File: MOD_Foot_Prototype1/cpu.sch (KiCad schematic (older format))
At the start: 19 parts, among them CN1 CONN_PANNEL_2X2, CN2 CONN_PANNEL_2X2, P1 HEADER_5X2, P2 HEADER_5X2, U1 LPC111X_LQFP48, X1 10MHz

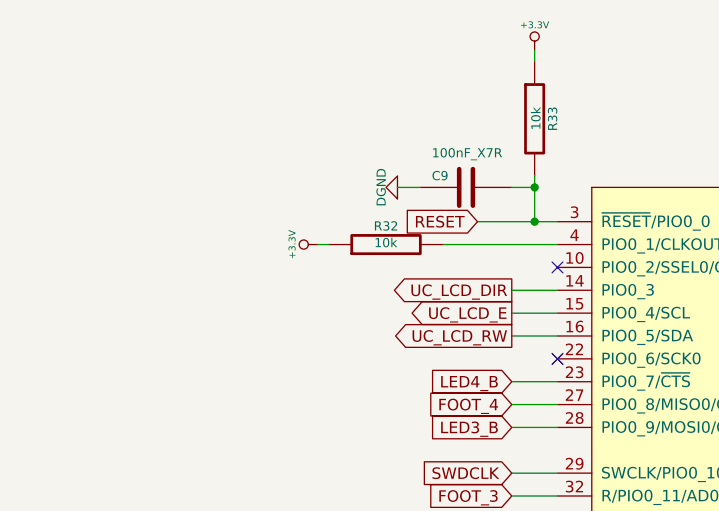
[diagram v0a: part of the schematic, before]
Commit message: add pull up resistors (to 3V3) to the LCD ENABLE and RW signals (wip issue #10)
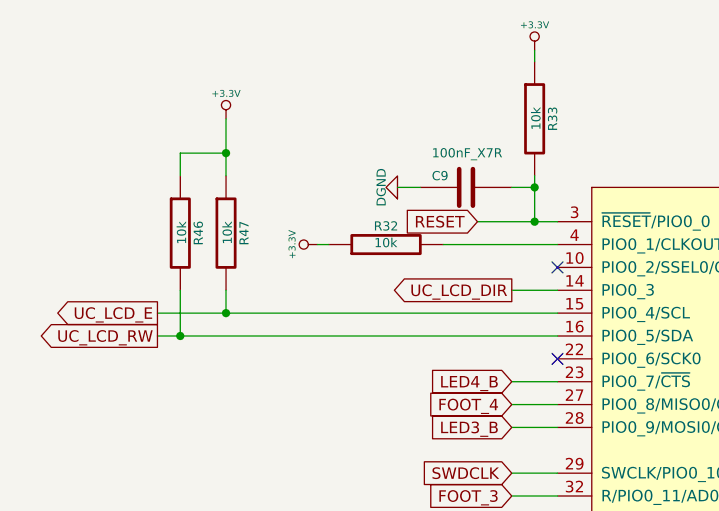
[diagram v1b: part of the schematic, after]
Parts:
- added R46, R47: 10k, MOD_Footprints_Lib:SM0603, symbol R
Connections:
- net +3.3V: now also R46.1, R47.1
- net UC_LCD_E: now also R47.2
- net UC_LCD_RW: now also R46.2
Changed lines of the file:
@@
 $EndComp
 $Comp
-L DGND #PWR30
+L DGND #PWR021
 U 1 1 54834712
 P 5550 4000
-F 0 "#PWR30" H 5550 4000 40  0001 C CNN
+F 0 "#PWR021" H 5550 4000 40  0001 C CNN
 F 1 "DGND" H 5550 3930 40  0000 C CNN
 F 2 "" H 5550 4000 60  0000 C CNN
@@
 $EndComp
 $Comp
-L DGND #PWR35
+L DGND #PWR022
 U 1 1 5483471F
 P 6550 3600
-F 0 "#PWR35" H 6550 3600 40  0001 C CNN
+F 0 "#PWR022" H 6550 3600 40  0001 C CNN
 F 1 "DGND" H 6550 3530 40  0000 C CNN
 F 2 "" H 6550 3600 60  0000 C CNN
@@
 $EndComp
 $Comp
-L DGND #PWR34
+L DGND #PWR023
 U 1 1 54834725
 P 6550 3400
-F 0 "#PWR34" H 6550 3400 40  0001 C CNN
+F 0 "#PWR023" H 6550 3400 40  0001 C CNN
 F 1 "DGND" H 6550 3330 40  0000 C CNN
 F 2 "" H 6550 3400 60  0000 C CNN
@@
 $EndComp
 $Comp
-L +3.3V #PWR31
+L +3.3V #PWR024
 U 1 1 5483472B
 P 5950 3350
-F 0 "#PWR31" H 5950 3310 30  0001 C CNN
+F 0 "#PWR024" H 5950 3310 30  0001 C CNN
 F 1 "+3.3V" H 5950 3460 30  0000 C CNN
 F 2 "" H 5950 3350 60  0000 C CNN
@@
 $EndComp
 $Comp
-L DGND #PWR33
+L DGND #PWR025
 U 1 1 5483473F
 P 6350 4900
-F 0 "#PWR33" H 6350 4900 40  0001 C CNN
+F 0 "#PWR025" H 6350 4900 40  0001 C CNN
 F 1 "DGND" H 6350 4830 40  0000 C CNN
 F 2 "" H 6350 4900 60  0000 C CNN
@@
 $EndComp
 $Comp
-L DGND #PWR32
+L DGND #PWR026
 U 1 1 54834745
 P 6350 4100
-F 0 "#PWR32" H 6350 4100 40  0001 C CNN
+F 0 "#PWR026" H 6350 4100 40  0001 C CNN
 F 1 "DGND" H 6350 4030 40  0000 C CNN
 F 2 "" H 6350 4100 60  0000 C CNN
@@
 $EndComp
 $Comp
-L DGND #PWR24
+L DGND #PWR027
 U 1 1 54834760
 P 2150 1400
-F 0 "#PWR24" H 2150 1400 40  0001 C CNN
+F 0 "#PWR027" H 2150 1400 40  0001 C CNN
 F 1 "DGND" H 2150 1330 40  0000 C CNN
 F 2 "" H 2150 1400 60  0000 C CNN
@@
 $EndComp
 $Comp
-L +3.3V #PWR26
+L +3.3V #PWR028
 U 1 1 54834766
 P 2750 800
-F 0 "#PWR26" H 2750 760 30  0001 C CNN
+F 0 "#PWR028" H 2750 760 30  0001 C CNN
 F 1 "+3.3V" H 2750 910 30  0000 C CNN
 F 2 "" H 2750 800 60  0000 C CNN
@@
 SWDCLK
 $Comp
-L DGND #PWR29
+L DGND #PWR029
 U 1 1 54834777
 P 4250 6450
-F 0 "#PWR29" H 4250 6450 40  0001 C CNN
+F 0 "#PWR029" H 4250 6450 40  0001 C CNN
 F 1 "DGND" H 4250 6380 40  0000 C CNN
 F 2 "" H 4250 6450 60  0000 C CNN
@@
 Text GLabel 2650 3950 0    50   Output ~ 0
 UC_LCD_RS
-Text GLabel 2650 2050 0    50   Output ~ 0
+Text GLabel 1100 2050 0    50   Output ~ 0
 UC_LCD_RW
 Text GLabel 5650 2300 2    50   Output ~ 0
 UC_LCD_BACK
-Text GLabel 2650 1950 0    50   Output ~ 0
+Text GLabel 1100 1950 0    50   Output ~ 0
 UC_LCD_E
 Text GLabel 2650 4150 0    50   Input ~ 0
@@
 TX_CHAIN
 $Comp
-L +5V #PWR21
+L +5V #PWR030
 U 1 1 5483479B
 P 1100 6400
-F 0 "#PWR21" H 1100 6490 20  0001 C CNN
+F 0 "#PWR030" H 1100 6490 20  0001 C CNN
 F 1 "+5V" H 1100 6490 30  0000 C CNN
 F 2 "" H 1100 6400 60  0000 C CNN
@@
 $EndComp
 $Comp
-L DGND #PWR22
+L DGND #PWR031
 U 1 1 548347A1
 P 1200 6300
-F 0 "#PWR22" H 1200 6300 40  0001 C CNN
+F 0 "#PWR031" H 1200 6300 40  0001 C CNN
 F 1 "DGND" H 1200 6225 40  0000 C CNN
 F 2 "" H 1200 6300 60  0000 C CNN
@@
 $EndComp
 $Comp
-L +3.3V #PWR23
+L +3.3V #PWR032
 U 1 1 548347AE
 P 1800 1650
-F 0 "#PWR23" H 1800 1610 30  0001 C CNN
+F 0 "#PWR032" H 1800 1610 30  0001 C CNN
 F 1 "+3.3V" H 1800 1760 30  0000 C CNN
 F 2 "" H 1800 1650 60  0000 C CNN
@@
 $EndComp
 $Comp
-L +3.3V #PWR28
+L +3.3V #PWR033
 U 1 1 54834827
 P 3750 5950
-F 0 "#PWR28" H 3750 5910 30  0001 C CNN
+F 0 "#PWR033" H 3750 5910 30  0001 C CNN
 F 1 "+3.3V" H 3750 6060 30  0000 C CNN
 F 2 "" H 3750 5950 60  0000 C CNN
@@
 NoConn ~ 5450 3300
 $Comp
-L DGND #PWR36
+L DGND #PWR034
 U 1 1 5483484A
 P 7350 5950
-F 0 "#PWR36" H 7350 5950 40  0001 C CNN
+F 0 "#PWR034" H 7350 5950 40  0001 C CNN
 F 1 "DGND" H 7350 5880 40  0000 C CNN
 F 2 "" H 7350 5950 60  0000 C CNN
@@
 $EndComp
 $Comp
-L DGND #PWR37
+L DGND #PWR035
 U 1 1 54834850
 P 8350 5950
-F 0 "#PWR37" H 8350 5950 40  0001 C CNN
+F 0 "#PWR035" H 8350 5950 40  0001 C CNN
 F 1 "DGND" H 8350 5880 40  0000 C CNN
 F 2 "" H 8350 5950 60  0000 C CNN
@@
 $EndComp
 $Comp
-L +5V #PWR27
+L +5V #PWR036
 U 1 1 548788DF
 P 2800 6400
-F 0 "#PWR27" H 2800 6490 20  0001 C CNN
+F 0 "#PWR036" H 2800 6490 20  0001 C CNN
 F 1 "+5V" H 2800 6490 30  0000 C CNN
 F 2 "" H 2800 6400 60  0000 C CNN
@@
 $EndComp
 $Comp
-L DGND #PWR25
+L DGND #PWR037
 U 1 1 548788E5
 P 2700 6300
-F 0 "#PWR25" H 2700 6300 40  0001 C CNN
+F 0 "#PWR037" H 2700 6300 40  0001 C CNN
 F 1 "DGND" H 2700 6225 40  0000 C CNN
 F 2 "" H 2700 6300 60  0000 C CNN
@@
 	2650 1850 2850 1850
 Wire Wire Line
-	2650 1950 2850 1950
-Wire Wire Line
-	2650 2050 2850 2050
+	1100 1950 2850 1950
+Wire Wire Line
+	1100 2050 2850 2050
 Wire Wire Line
 	2650 3450 2850 3450
@@
 	2400 6050 2200 6050
 Connection ~ 2400 6700
+$Comp
+L R R46
+U 1 1 54908ABC
+P 1200 1600
+F 0 "R46" V 1280 1600 40  0000 C CNN
+F 1 "10k" V 1207 1601 40  0000 C CNN
+F 2 "MOD_Footprints_Lib:SM0603" V 1130 1600 30  0001 C CNN
+F 3 "~" H 1200 1600 30  0000 C CNN
+	1    1200 1600
+	1    0    0    -1
+$EndComp
+$Comp
+L R R47
+U 1 1 54908B10
+P 1400 1600
+F 0 "R47" V 1480 1600 40  0000 C CNN
+F 1 "10k" V 1407 1601 40  0000 C CNN
+F 2 "MOD_Footprints_Lib:SM0603" V 1330 1600 30  0001 C CNN
+F 3 "~" H 1400 1600 30  0000 C CNN
+	1    1400 1600
+	1    0    0    -1
+$EndComp
+Wire Wire Line
+	1200 1350 1200 1250
+Wire Wire Line
+	1200 1250 1400 1250
+Wire Wire Line
+	1400 1100 1400 1350
+Wire Wire Line
+	1200 1850 1200 2050
+Connection ~ 1200 2050
+Wire Wire Line
+	1400 1850 1400 1950
+Connection ~ 1400 1950
+$Comp
+L +3.3V #PWR038
+U 1 1 54908FE8
+P 1400 1100
+F 0 "#PWR038" H 1400 1060 30  0001 C CNN
+F 1 "+3.3V" H 1400 1210 30  0000 C CNN
+F 2 "" H 1400 1100 60  0000 C CNN
+F 3 "" H 1400 1100 60  0000 C CNN
+	1    1400 1100
+	1    0    0    -1
+$EndComp
+Connection ~ 1400 1250
 $EndSCHEMATC
